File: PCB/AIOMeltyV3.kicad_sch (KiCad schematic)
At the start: 30 parts, among them J1 USB4500-03-0-A_REVA1, SW1 Boot, SW2 Reset, U3 ESP32-S3-MINI-1, U4 RT9161A-33GV

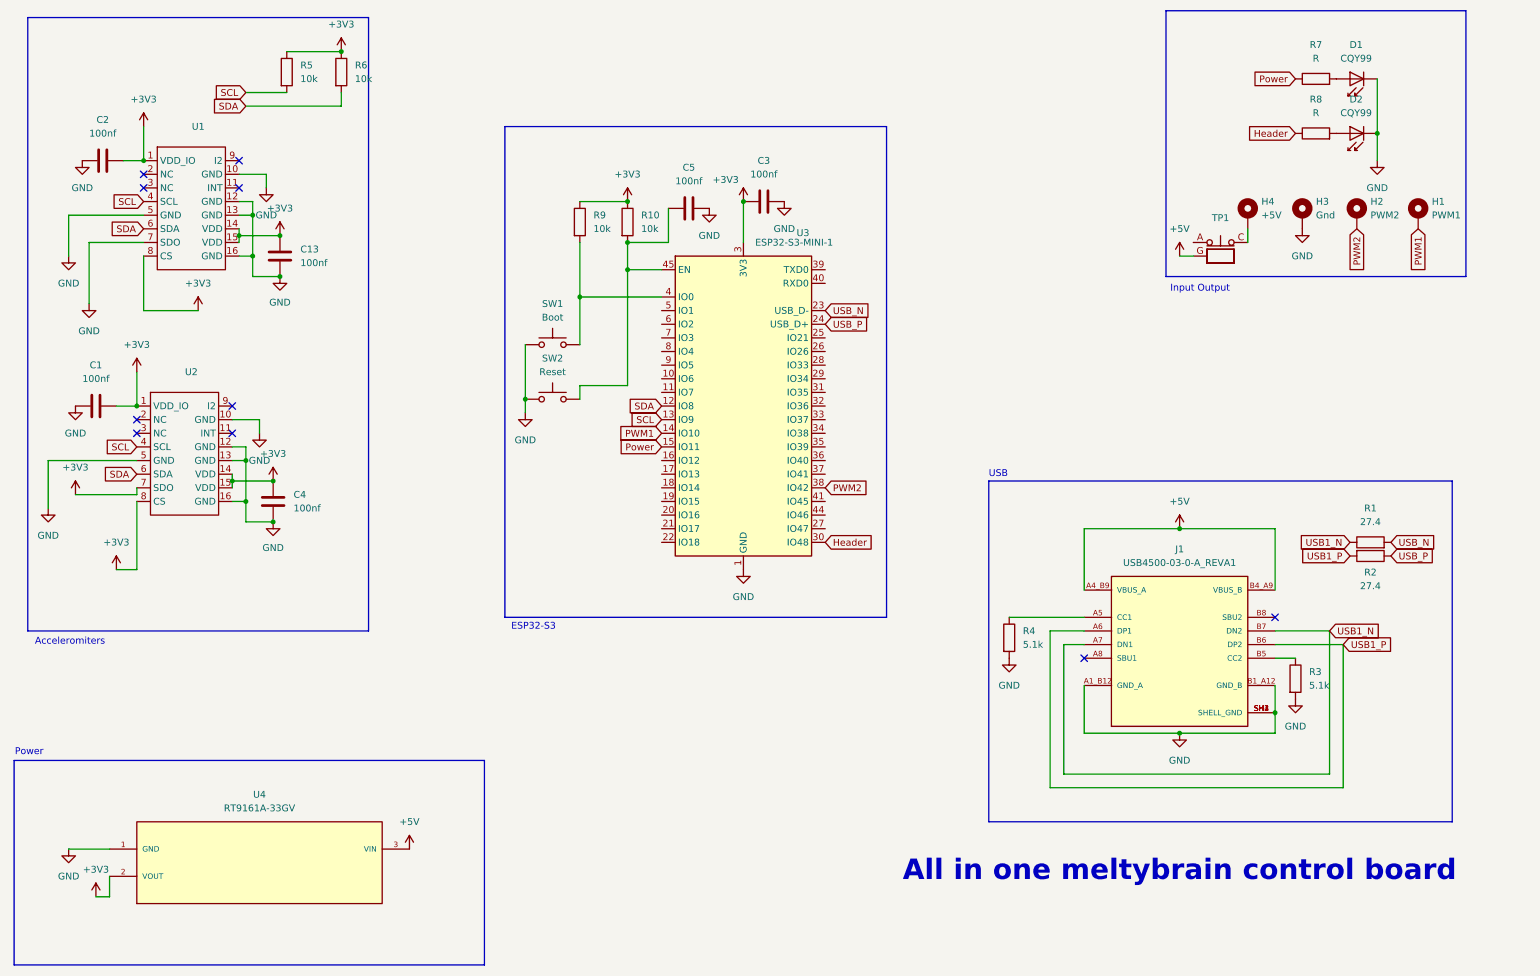
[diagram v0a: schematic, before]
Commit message: I belive this is PIO updating librarys
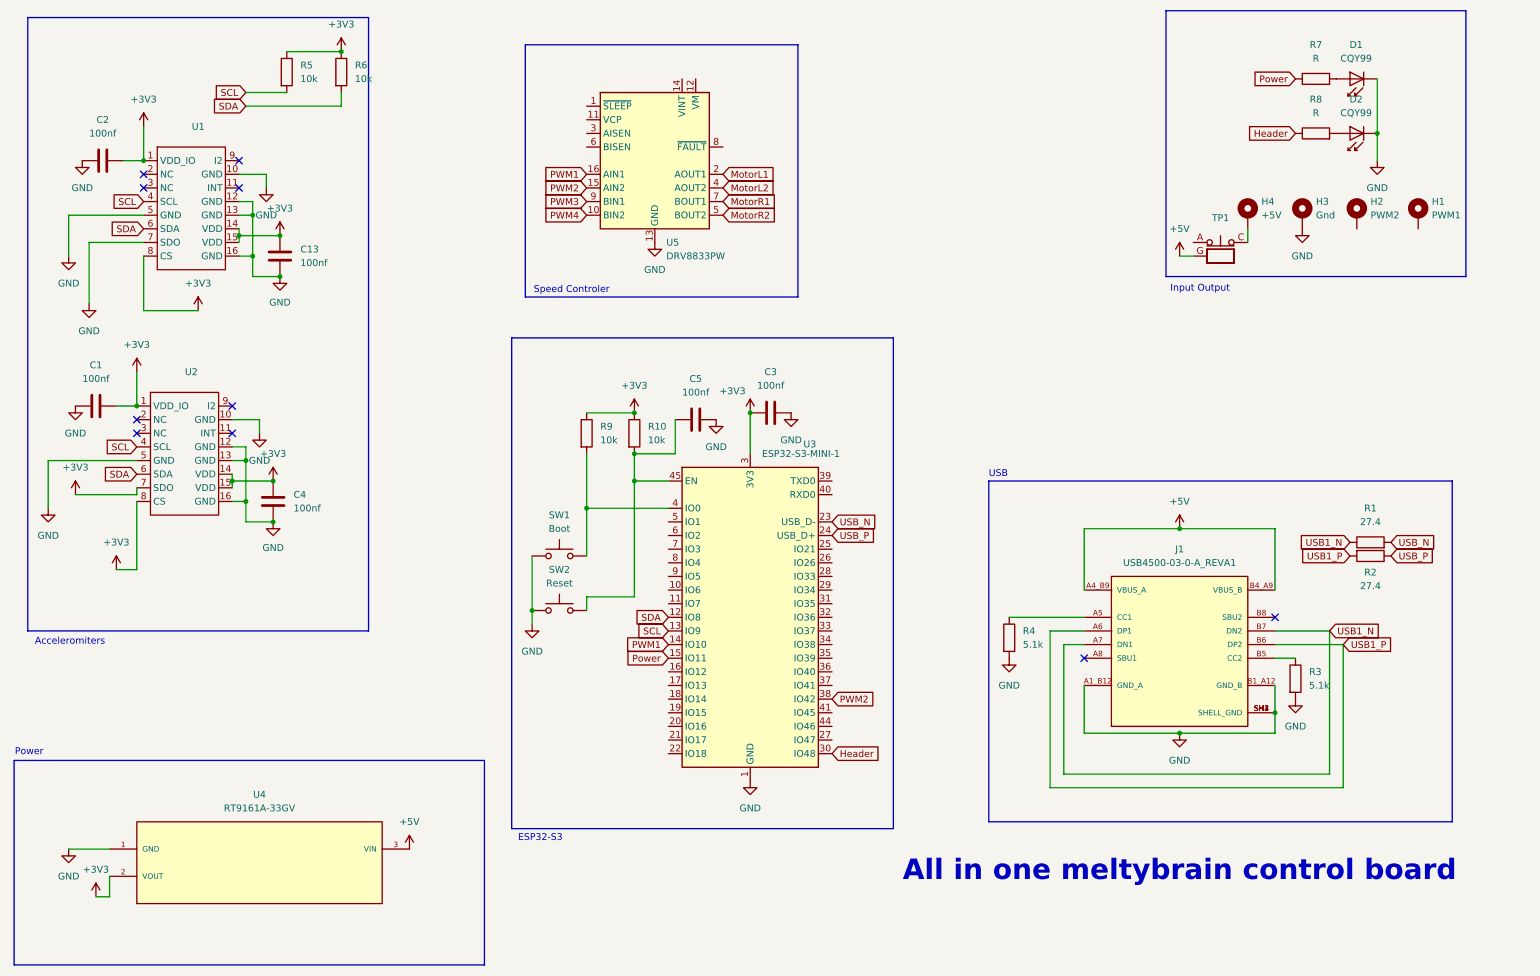
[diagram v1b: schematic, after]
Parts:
- added U5: DRV8833PW, Package_SO:TSSOP-16_4.4x5mm_P0.65mm, symbol Driver_Motor:DRV8833PW
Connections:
- net GND: now also U5.13 (GND)
- net PWM1: now also U5.16 (AIN1); no longer H1.MP
- net PWM2: now also U5.15 (AIN2); no longer H2.MP
- new net MotorL1: U5.2 (AOUT1)
- new net MotorL2: U5.4 (AOUT2)
- new net MotorR1: U5.7 (BOUT1)
- new net MotorR2: U5.5 (BOUT2)
- new net PWM3: U5.9 (BIN1)
- new net PWM4: U5.10 (BIN2)
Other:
- note added: "Speed Controler"
- moved on the sheet: C3, C5, R10, R9, SW1, SW2, U3
